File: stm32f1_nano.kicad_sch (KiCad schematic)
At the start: 48 parts, among them J1 Analog, J2 Digital, J3 TYPE-C-31-M-12, J4 Conn_ST_STDC14, Q1 AO3401A, Q3 AO3401A, U1 STM32F103C8T6, U2 W25Q32JVSS, U3 AMS1117-3.3, U5 AMS1117-5.0, X1 NX3225GD-8MHZ-STD-CRA-3

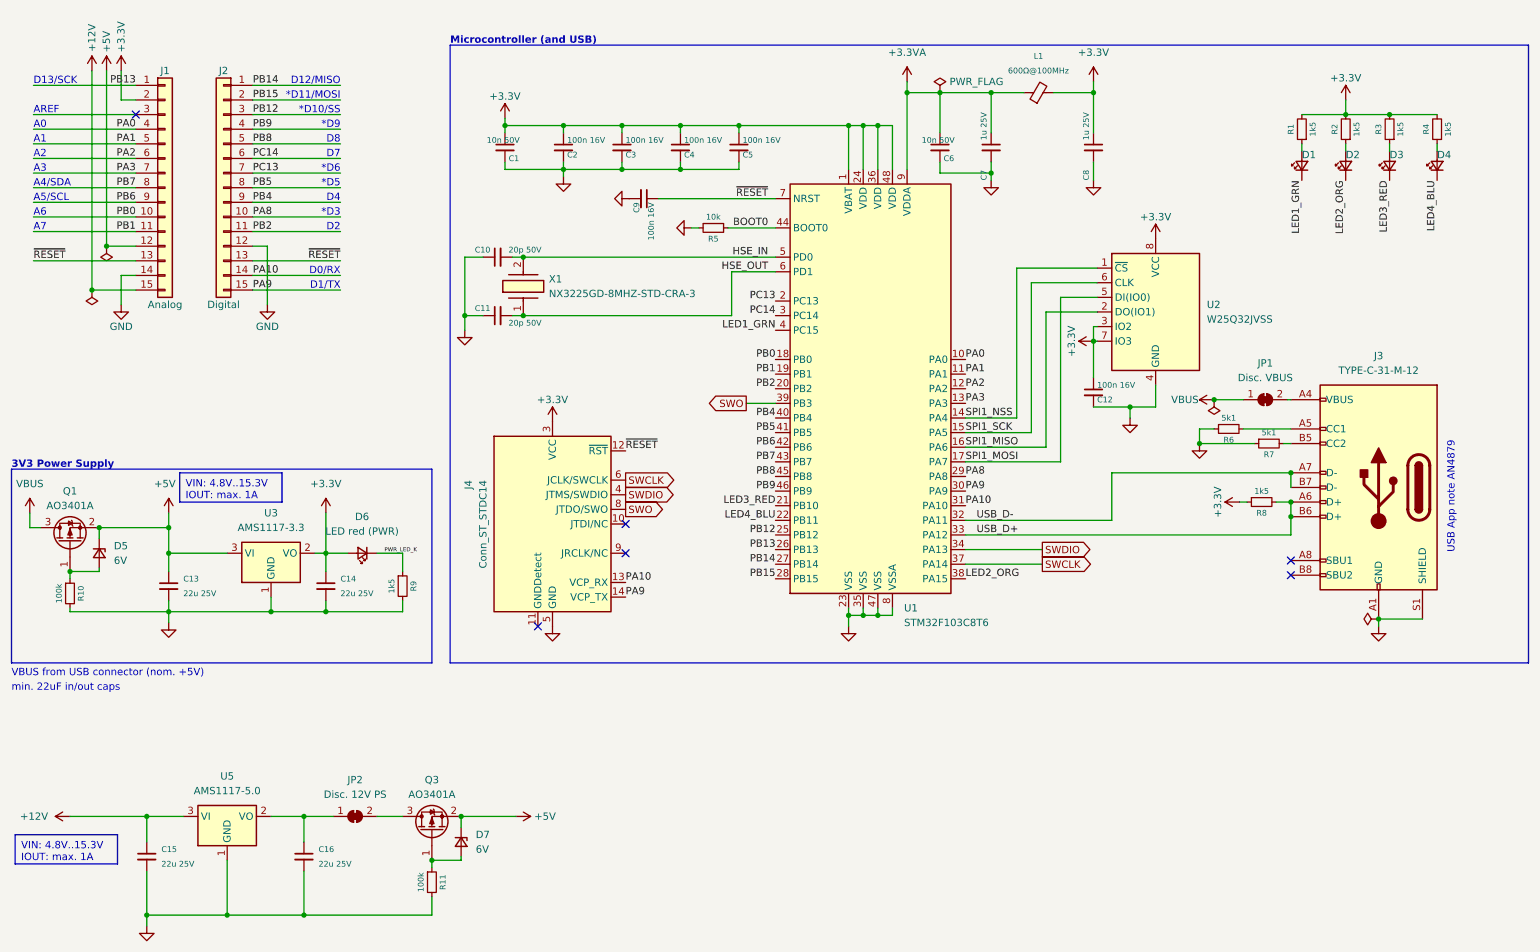
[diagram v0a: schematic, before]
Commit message: First draft almost done
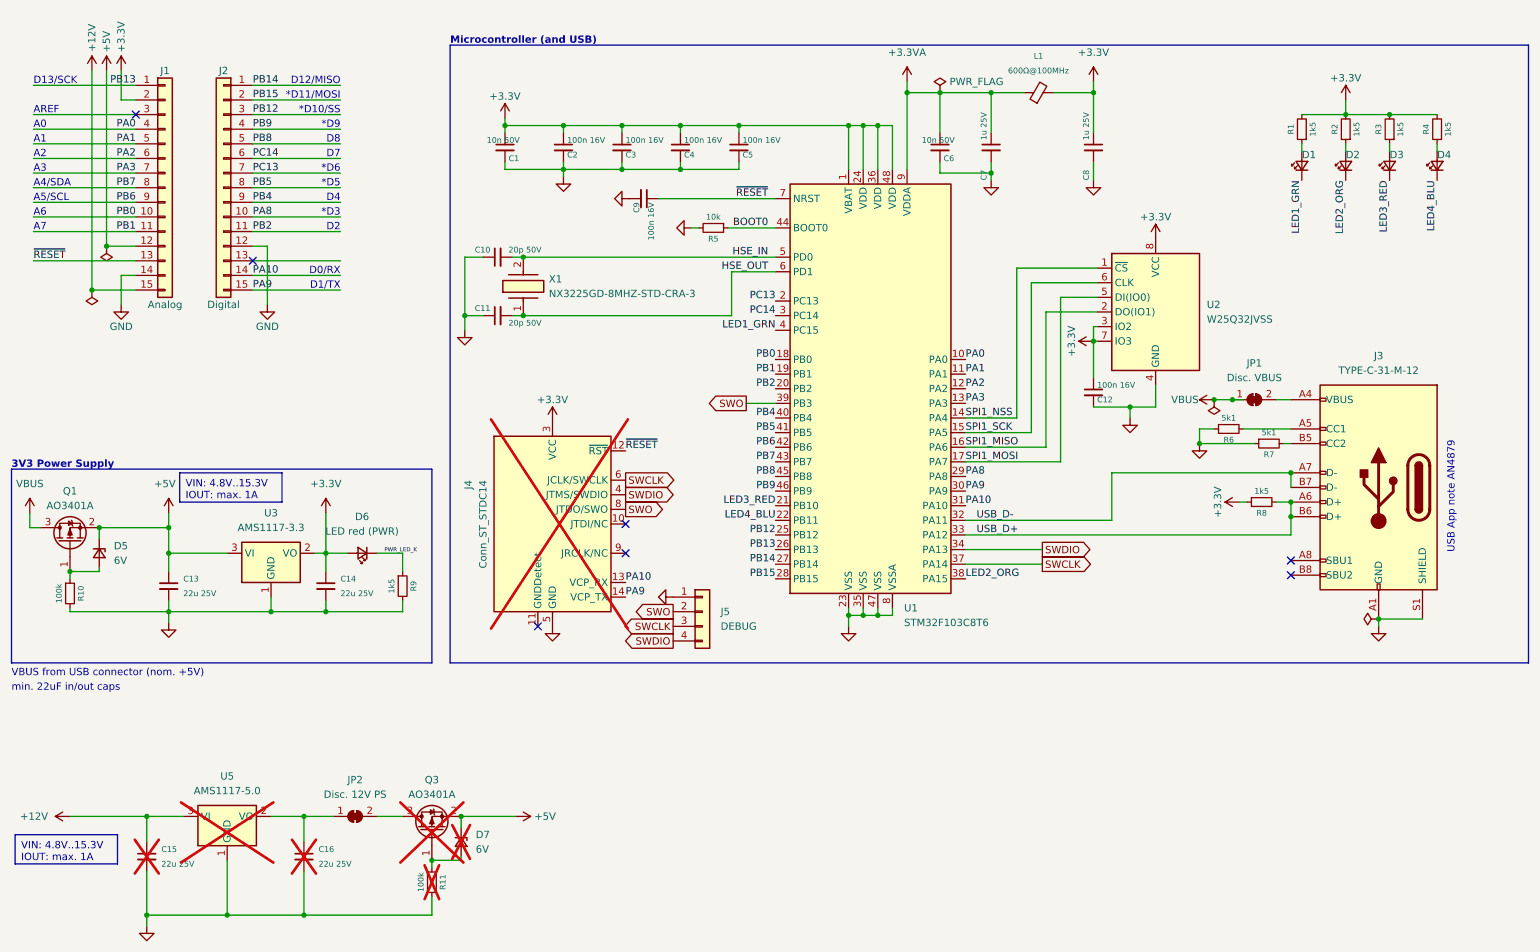
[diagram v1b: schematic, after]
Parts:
- added J5: DEBUG, Connector_PinHeader_2.54mm:PinHeader_1x04_P2.54mm_Vertical, symbol Connector_Generic:Conn_01x04
- C15, C16, D7, J4, Q3, R11, U5: now not fitted
- J1, J2: now left out of the parts list
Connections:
- net GND: now also J5.1 (Pin_1)
- net SWCLK: now also J5.3 (Pin_3)
- net SWDIO: now also J5.4 (Pin_4)
- net SWO: now also J5.2 (Pin_2)
- net ~{RESET}: no longer J2.13 (Pin_13)
- no-connect marks 6 -> 7
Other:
- moved on the sheet: JP1
